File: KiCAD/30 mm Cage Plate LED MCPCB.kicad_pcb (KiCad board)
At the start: 2 copper layers, 40 x 40 mm, 13 parts, among them IC1 AL8843QSP-13, J1 Conn_01x04

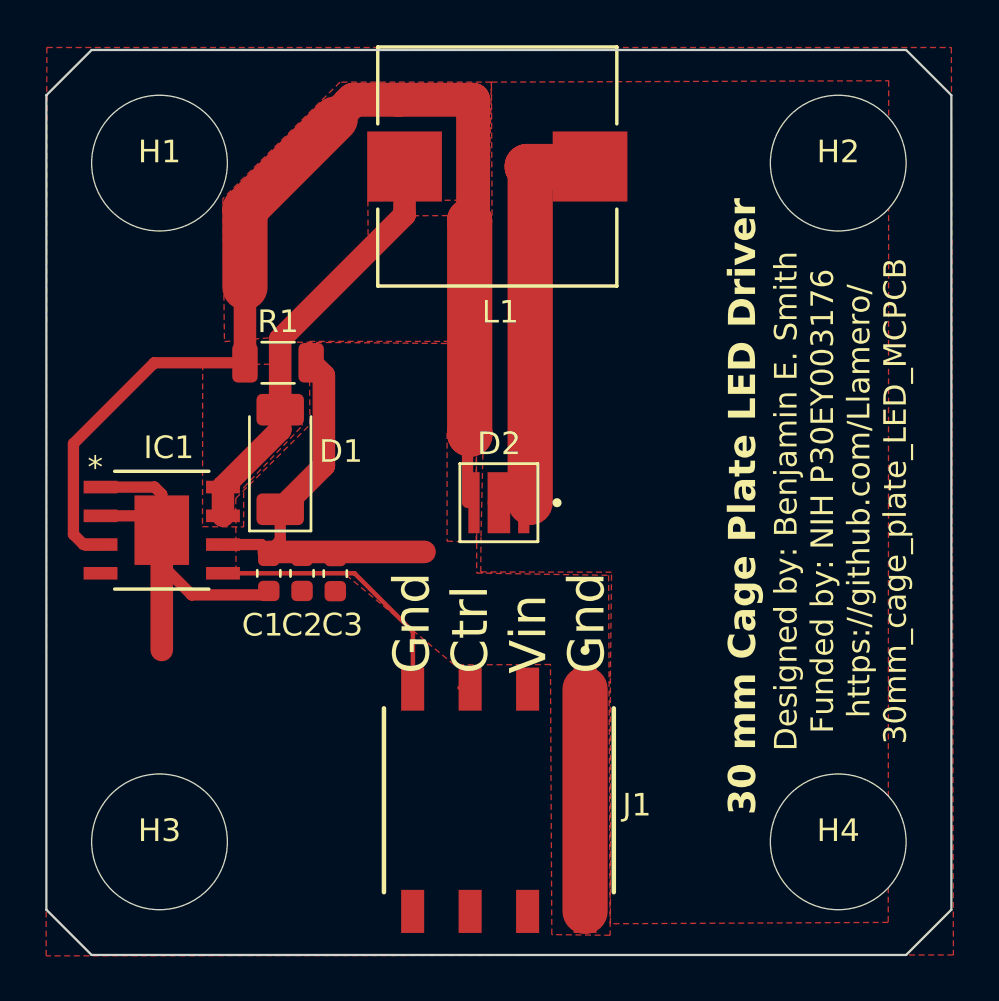
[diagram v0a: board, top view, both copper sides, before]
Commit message: working draft
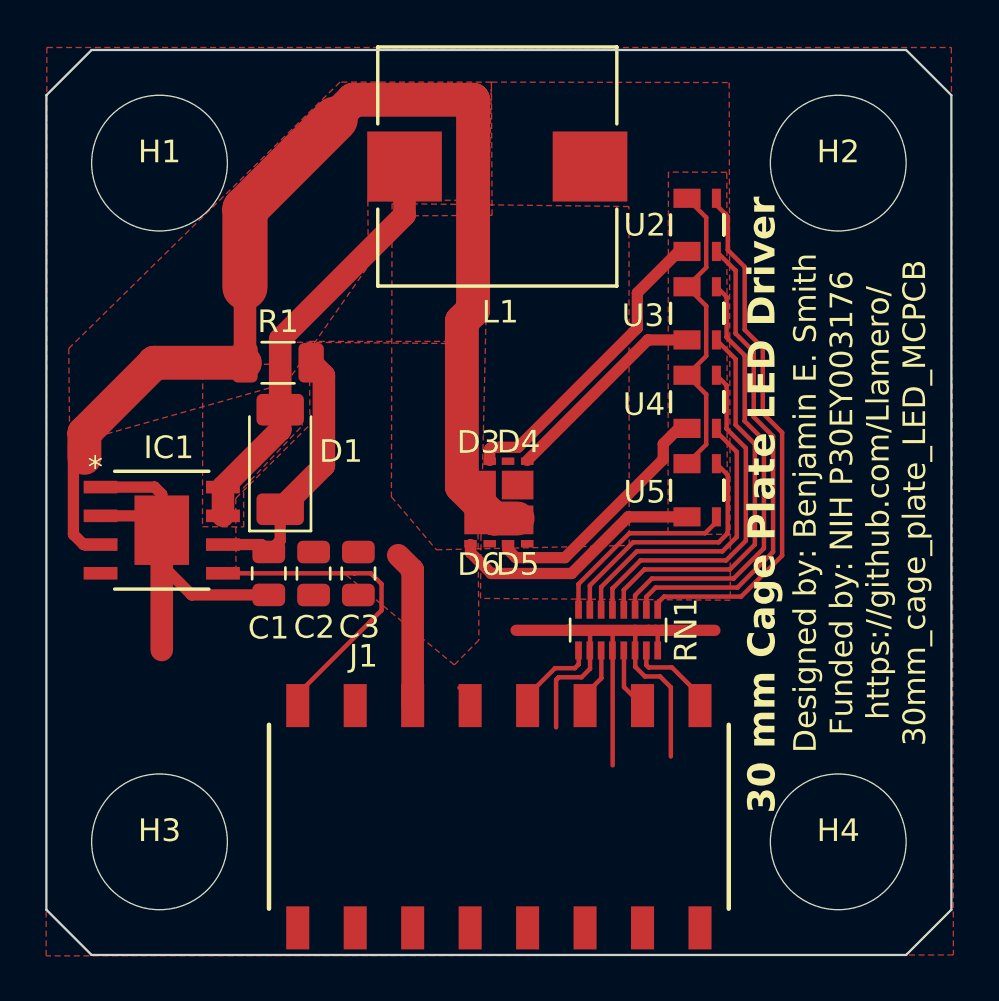
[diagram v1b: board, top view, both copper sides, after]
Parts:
- removed D2: SST-10-IRD-B90H-S810, Custom:LED_SST-10-IRD-B90H-S810
- added D3: LED_Pad, Custom:LED_XLAMP_XE-G_CRW, F.Cu at (119.2, 78.9)
- added D4: LED_Pad, Custom:LED_XLAMP_XE-G_CRW, F.Cu at (120.8, 78.9)
- added D5: LED_Pad, Custom:LED_XLAMP_XE-G_CRW, F.Cu at (120.8, 81.1)
- added D6: LED_Pad, Custom:LED_XLAMP_XE-G_CRW, F.Cu at (119.2, 81.1)
- added RN1: 180, Resistor_SMD:R_Array_Convex_8x0602, F.Cu at (125.3, 85.6)
- added U2: TLP3480, Custom:TLP3480-SSR, F.Cu at (128.8, 67.7)
- added U3: TLP3480, Custom:TLP3480-SSR, F.Cu at (128.8, 71.6)
- added U4: TLP3480, Custom:TLP3480-SSR, F.Cu at (128.8, 75.5)
- added U5: TLP3480, Custom:TLP3480-SSR, F.Cu at (128.8, 79.5)
- C1, C2, C3: value 10μF -> 22μF; footprint Capacitor_SMD:C_0603_1608Metric -> Capacitor_SMD:C_0805_2012Metric
- J1: value Conn_01x04 -> Conn_01x08_Socket; footprint Custom:SAMTEC_SSM-104-L-SH -> Custom:SAMTEC_SSM-108-F-SH-TR
- R1: value 0.068 -> 0.040
- moved C3 1.02 mm to (113.8, 83.1)
- moved J1 0.73 mm to (120.0, 93.9), turned to 0 degrees
- moved C2 0.51 mm to (111.8, 83.1)
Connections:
- net Net-(IC1-SET) renamed /LED+
- J1 pad 1: /Vin -> /PWM
- J1 pad 3: GND -> /Vin
- J1 pad 4: /PWM -> GND
- L1 pad 1: Net-(D2-PadC) -> /LED-
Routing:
- net GND: track 20.5 -> 48.3 mm
- net Net-(RN1-R1.1): track 0.00 -> 23.7 mm
- net Net-(D2-PadC): track 21.7 -> 0.00 mm
- net Net-(RN1-R2.1): track 0.00 -> 21.3 mm
- net Net-(RN1-R3.1): track 0.00 -> 19.6 mm
- net Net-(RN1-R4.1): track 0.00 -> 17.2 mm
- net Net-(RN1-R5.1): track 0.00 -> 15.6 mm
- net /LED-: track 0.00 -> 13.8 mm
- net Net-(D3-K): track 0.00 -> 13.8 mm
- net Net-(RN1-R6.1): track 0.00 -> 13.1 mm
- net Net-(RN1-R7.1): track 0.00 -> 11.4 mm
- net Net-(D6-K): track 0.00 -> 11.4 mm
- net Net-(D5-K): track 0.00 -> 11.0 mm
- net /Vin: track 28.5 -> 18.7 mm
- net Net-(D4-K): track 0.00 -> 9.27 mm
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- added copper zone on F.Cu, net /LED-
- removed copper zone on F.Cu, net Net-(D2-PadC)
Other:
- board text removed: "Gnd Ctrl Vin Gnd"
